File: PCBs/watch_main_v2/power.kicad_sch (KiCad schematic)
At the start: 22 parts, among them IC201 ADP5360ACBZ-2-R7, Q201 DMP2104LP-7

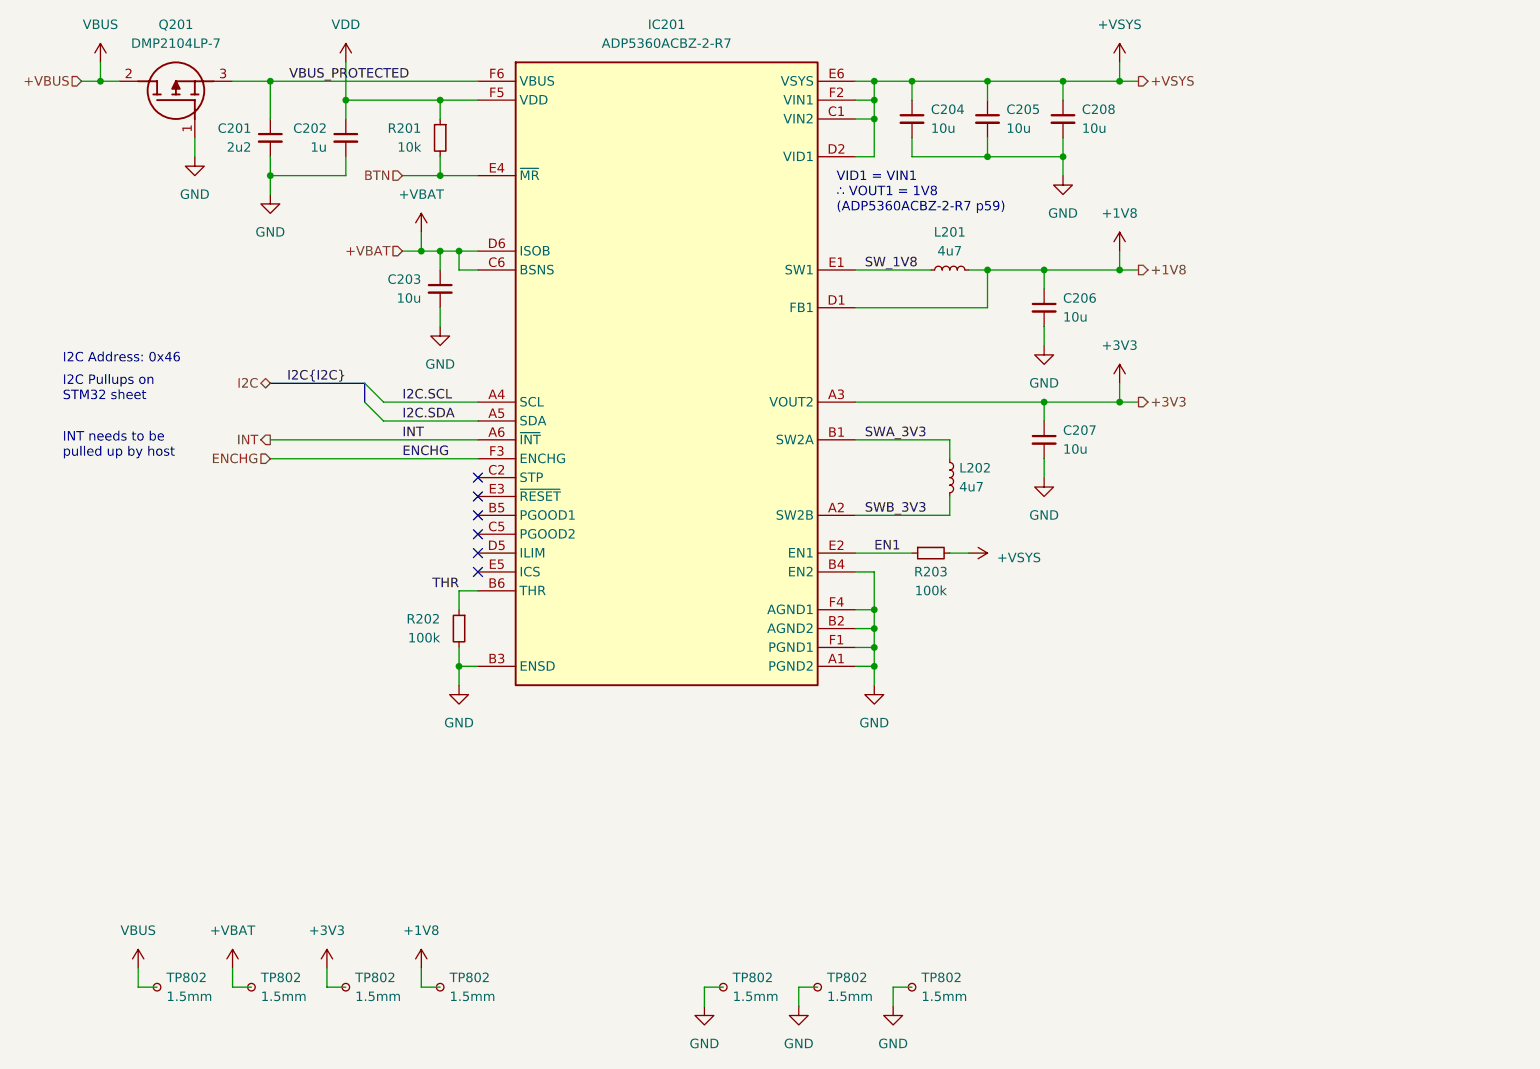
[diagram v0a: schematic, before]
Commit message: 190 Unrouted traces
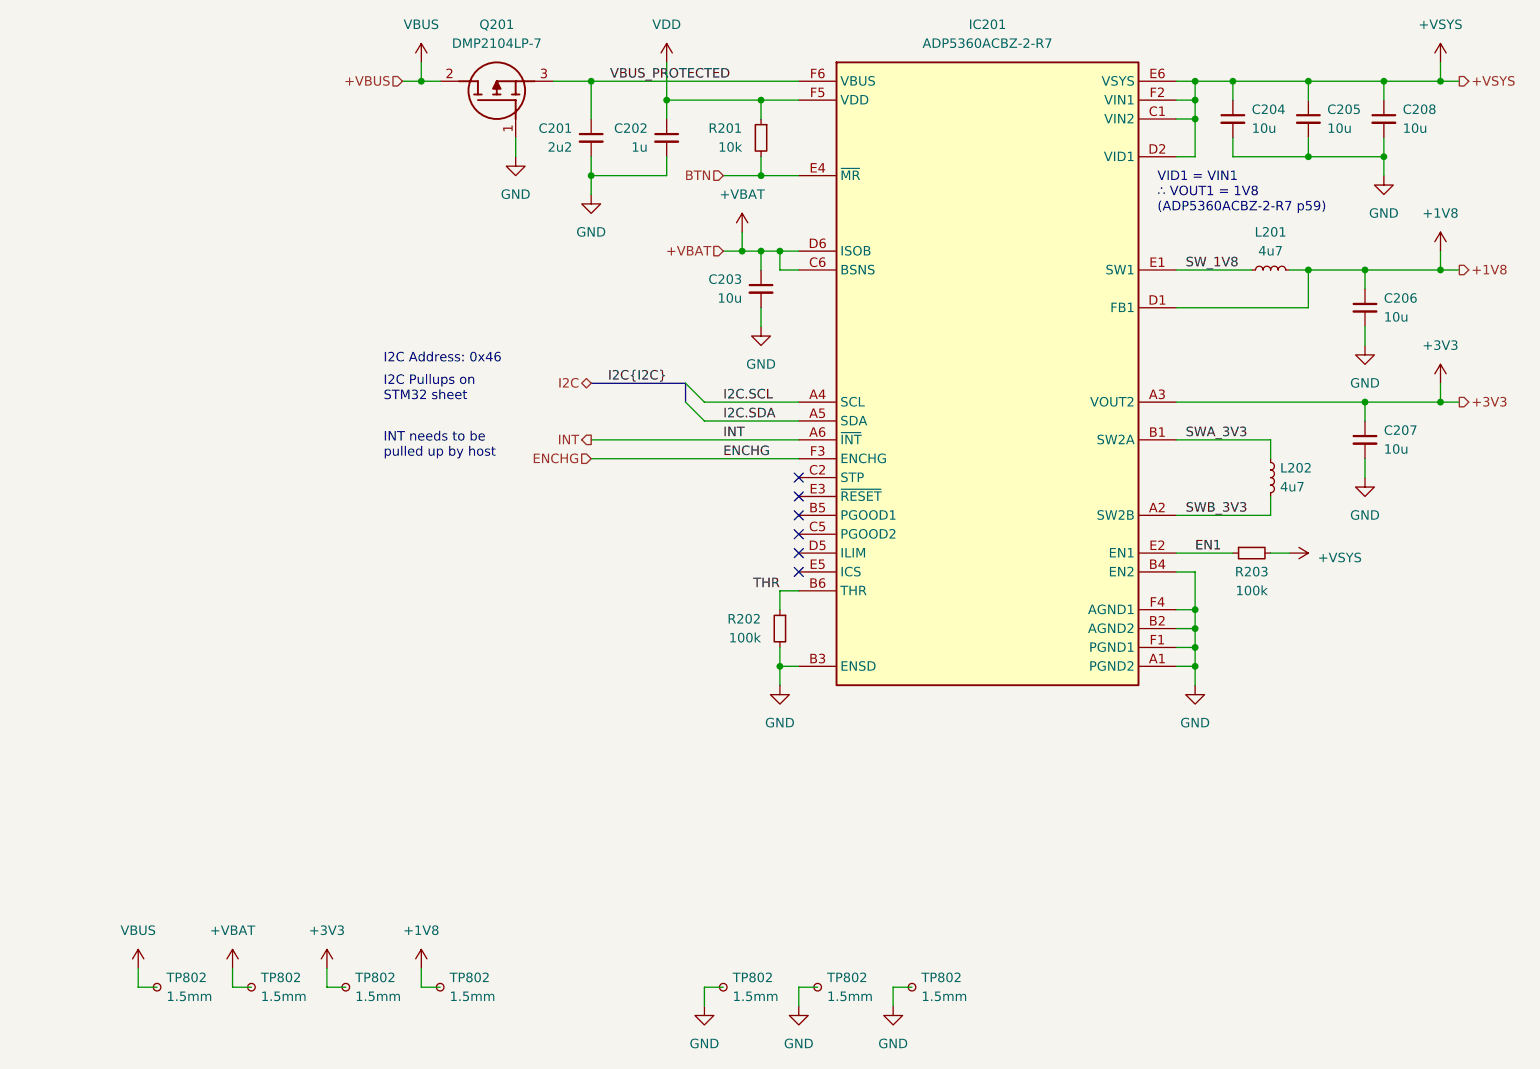
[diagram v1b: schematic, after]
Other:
- moved on the sheet: C201, C202, C203, C204, C205, C206, C207, C208, IC201, L201, L202, Q201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

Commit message: Main board v2 complete
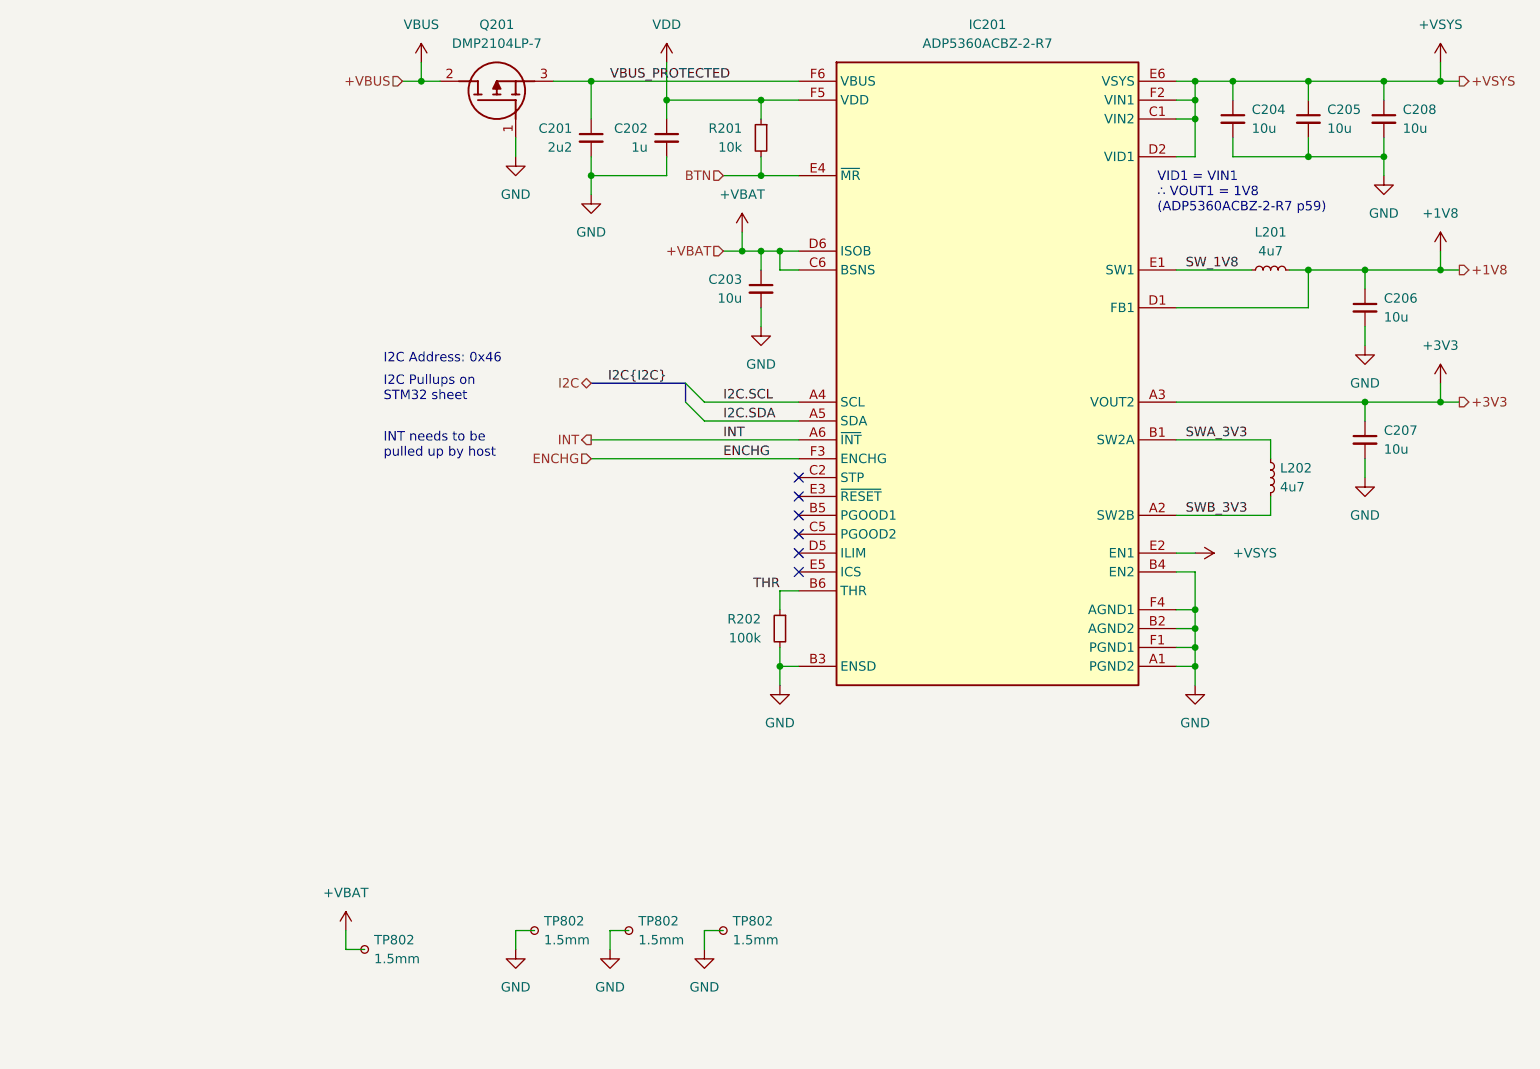
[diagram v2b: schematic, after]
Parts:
- removed R203: 100k, Resistor_SMD:R_0402_1005Metric, symbol Device:R_Small
- removed TP802 (x4): 1.5mm, TestPoint:TestPoint_Pad_D1.5mm, symbol Connector:TestPoint_Small
- added TP802: 1.5mm, TestPoint:TestPoint_Pad_D1.5mm, symbol Connector:TestPoint_Small
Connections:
- net EN1 is gone; now on net +VSYS: IC201.E2 (EN1)
- net GND: now also TP802.1
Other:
- moved on the sheet: TP802
